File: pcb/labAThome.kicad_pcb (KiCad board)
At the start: 2 copper layers, 100 x 100 mm, 119 parts, among them IC1 MD8002A, J1 I2C, J10 SPK, J11 24.5.GND.3, J12 NEOPIXEL, J13 Power Input 1, J14 Conn_Coaxial, J15 WS2812_OUT, J16 HCP, J2 SRVx, J3 5V, J4 EXT, J5 VPS, J6 FAN2, J7 1wire, J8 1wire, J9 FAN1, K1 G5V-2, K2 G5V-2, K3 G5V-2, M3 SN65HVD230_MODULE, Q1 BC847, Q2 IRLZ44N, Q3 IRLML6344, Q4 BC847, Q5 IRF530, Q6 IRLML5203, SW1 RED, SW2 GREEN, SW4 BLUE, SW5 WHITE, SW7 ROTENC, U1 SR602, U10 MAX3485_MODULE, U11 AM312, U12 24V->4V, U13 LM358, U14 MS4525DO, U15 CCS811_MODULE, U16 24V->5V, U17 DS18B20, U2 TPS5430DDA, U3 Power Input 2, U4 ESP32_DEVKITC_COMPATIBLE, U6 GY-302, U7 Display, U8 MIC, U9 RFM95W-868S2, X1 FAN_6024, m1 Attribution

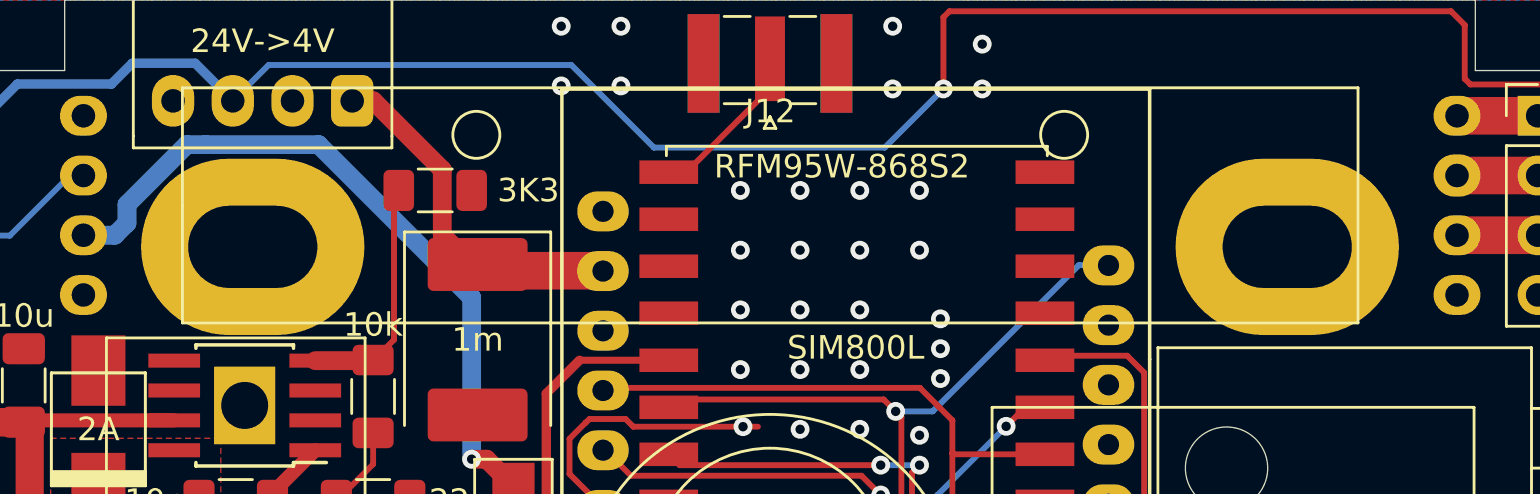
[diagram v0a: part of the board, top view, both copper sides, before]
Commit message: pcb V10 as ordered at JLCPCB
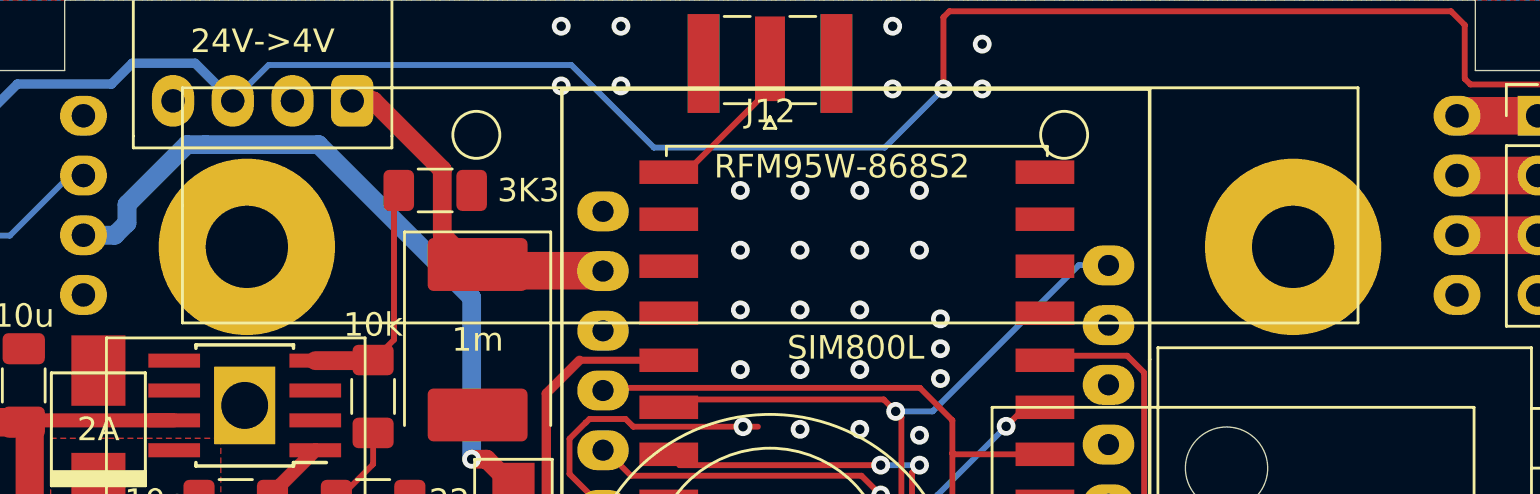
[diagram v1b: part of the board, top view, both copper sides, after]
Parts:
- R11: footprint smopla:Resistor_100W -> liebler_PASSIVES:Resistor_100W
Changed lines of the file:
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@@
     (34 B.Paste user hide)
     (35 F.Paste user hide)
-    (36 B.SilkS user hide)
+    (36 B.SilkS user)
     (37 F.SilkS user)
     (38 B.Mask user hide)
@@
   )
   (setup
-    (last_trace_width 0.4)
+    (last_trace_width 0.25)
     (user_trace_width 0.3)
     (user_trace_width 0.4)
@@
     (add_net /Q2_D)
   )
+  (module liebler_PASSIVES:Resistor_100W (layer B.Cu)
+    (at 80 50.5)
+    (fp_text reference R11 (at -27.5 3.5) (layer B.SilkS) hide
+      (effects (font (size 1 1) (thickness 0.15)) (justify mirror))
+    )
+    (fp_text value "22R, 100W" (at 0 0) (layer B.SilkS)
+      (effects (font (size 4 4) (thickness 0.5)) (justify mirror))
+    )
+    (fp_line (start -30 4.5) (end 30 4.5) (layer B.SilkS) (width 0.12))
+    (fp_line (start 30 7.5) (end 30 -13.5) (layer B.SilkS) (width 0.12))
+    (fp_line (start 30 -13.5) (end -30 -13.5) (layer B.SilkS) (width 0.12))
+    (fp_line (start -30 -13.5) (end -30 7.5) (layer B.SilkS) (width 0.12))
+    (fp_line (start 30 0) (end 30 3) (layer B.SilkS) (width 0.12))
+    (fp_line (start 30 6.5) (end -30 6.5) (layer B.SilkS) (width 0.12))
+    (fp_line (start -30 7.5) (end 30 7.5) (layer B.SilkS) (width 0.12))
+    (fp_line (start 30 5.5) (end -30 5.5) (layer B.SilkS) (width 0.12))
+    (fp_line (start -30 -6.5) (end 30 -6.5) (layer B.SilkS) (width 0.12))
+    (fp_line (start -30 -7.5) (end 30 -7.5) (layer B.SilkS) (width 0.12))
+    (fp_line (start 30 2) (end 38 2) (layer B.SilkS) (width 0.12))
+    (fp_line (start 38 -2) (end 30 -2) (layer B.SilkS) (width 0.12))
+    (fp_line (start -30 -2) (end -38 -2) (layer B.SilkS) (width 0.12))
+    (fp_line (start -38 2) (end -30 2) (layer B.SilkS) (width 0.12))
+    (fp_line (start -30 -5.5) (end 30 -5.5) (layer B.SilkS) (width 0.12))
+    (fp_line (start -30 -4.5) (end 30 -4.5) (layer B.SilkS) (width 0.12))
+    (pad 2 thru_hole circle (at 39.7 0) (size 3.6 3.6) (drill 1.6) (layers *.Cu *.Mask)
+      (net 49 /Q2_D))
+    (pad 1 thru_hole circle (at -39.7 0) (size 3.6 3.6) (drill 1.6) (layers *.Cu *.Mask)
+      (net 2 +24V))
+    (pad "" np_thru_hole oval (at -22.25 -10) (size 7.5 7.5) (drill oval 3.5) (layers *.Cu *.Mask))
+    (pad "" np_thru_hole oval (at 22.25 -10) (size 7.5 7.5) (drill oval 3.5) (layers *.Cu *.Mask))
+    (model "${CUSTOM_LIBS}/smopla.3d/Resistor 100W.stp"
+      (offset (xyz 30 0 27.5))
+      (scale (xyz 1 1 1))
+      (rotate (xyz -90 0 90))
+    )
+    (model "${CUSTOM_LIBS}/smopla.3d/Resistor 100W.stp"
+      (offset (xyz 30 0 49.5))
+      (scale (xyz 1 1 1))
+      (rotate (xyz -90 0 90))
+    )
+  )
   (module liebler_MODULES:PIR_Sensor_SR602 (layer F.Cu)
     (at 80 55.626)
@@
       (effects (font (size 1 1) (thickness 0.15)))
     )
+    (fp_circle (center 0 0) (end 0 -8) (layer F.SilkS) (width 0.12))
+    (fp_circle (center 0 0) (end 0 -8) (layer F.CrtYd) (width 0.12))
     (fp_arc (start 8 0) (end 7.750001 -1.749999) (angle -163.7397953) (layer F.SilkS) (width 0.12))
     (fp_arc (start -8 0) (end -7.750001 1.749999) (angle -164.7448813) (layer F.SilkS) (width 0.12))
-    (fp_circle (center 0 0) (end 0 -8) (layer F.SilkS) (width 0.12))
-    (fp_circle (center 0 0) (end 0 -8) (layer F.CrtYd) (width 0.12))
     (pad 3 thru_hole circle (at 2.54 6.096) (size 1.8 1.8) (drill 1) (layers *.Cu *.Mask)
       (net 38 MOVEMENT))
@@
     (fp_text value ESP32_DEVKITC_COMPATIBLE (at 0 1.5) (layer F.Fab)
       (effects (font (size 1 1) (thickness 0.15)))
-    )
-    (fp_text user "WIFI ANTENNA" (at 0 -24) (layer F.SilkS)
-      (effects (font (size 2 1.5) (thickness 0.15)))
-    )
-    (fp_text user USB (at 0 24) (layer F.SilkS)
-      (effects (font (size 2 1.5) (thickness 0.15)))
     )
     (fp_line (start 0 -27.5) (end 14 -27.5) (layer F.SilkS) (width 0.12))
@@
     (fp_line (start 14 -27.5) (end -14 -27.5) (layer F.CrtYd) (width 0.12))
     (fp_line (start -14 -27.5) (end -14 27.5) (layer F.CrtYd) (width 0.12))
+    (fp_text user "WIFI ANTENNA" (at 0 -24) (layer F.SilkS)
+      (effects (font (size 2 1.5) (thickness 0.15)))
+    )
+    (fp_text user USB (at 0 24) (layer F.SilkS)
+      (effects (font (size 2 1.5) (thickness 0.15)))
+    )
     (pad 38 thru_hole circle (at 12.7 -22.86) (size 1.7 1.7) (drill 1) (layers *.Cu *.Mask)
       (net 1 GND))
@@
       (effects (font (size 1 1) (thickness 0.15)))
     )
-    (fp_text user %R (at 3.6 3.8 90) (layer F.Fab) hide
-      (effects (font (size 1 1) (thickness 0.15)))
-    )
     (fp_line (start -0.5 0) (end 0.5 0) (layer F.SilkS) (width 0.12))
     (fp_line (start 0 -0.5) (end 0 0.5) (layer F.SilkS) (width 0.12))
@@
     (fp_line (start -8.516 -3.516) (end -6.103 -3.516) (layer F.CrtYd) (width 0.12))
     (fp_line (start -6.103 -3.516) (end -6.103 -5.929) (layer F.CrtYd) (width 0.12))
+    (fp_text user %R (at 3.6 3.8 90) (layer F.Fab) hide
+      (effects (font (size 1 1) (thickness 0.15)))
+    )
     (pad A thru_hole roundrect (at -7.5 -2.5 270) (size 2 1.6) (drill 1) (layers *.Cu *.Mask) (roundrect_rratio 0.25)
       (net 57 ROTENC_A))
@@
     )
     (fp_text value WHITE (at 4.75 -7.25) (layer F.SilkS)
-      (effects (font (size 1 1) (thickness 0.15)))
-    )
-    (fp_text user %R (at 0.1 0.04) (layer F.Fab) hide
       (effects (font (size 1 1) (thickness 0.15)))
     )
@@
     (fp_line (start 6.15 3.43) (end 6.15 6.15) (layer F.SilkS) (width 0.12))
     (fp_line (start 6.15 -6.15) (end 6.15 -3.43) (layer F.SilkS) (width 0.12))
+    (fp_text user %R (at 0.1 0.04) (layer F.Fab) hide
+      (effects (font (size 1 1) (thickness 0.15)))
+    )
     (pad 2 thru_hole oval (at -6.25 2.5 180) (size 3.048 1.85) (drill 1.3) (layers *.Cu *.Mask)
       (net 6 +5V))
@@
     )
     (fp_text value BLUE (at -0.25 7) (layer F.SilkS)
-      (effects (font (size 1 1) (thickness 0.15)))
-    )
-    (fp_text user %R (at 0.1 0.04) (layer F.Fab) hide
       (effects (font (size 1 1) (thickness 0.15)))
     )
@@
     (fp_line (start 6.15 3.43) (end 6.15 6.15) (layer F.SilkS) (width 0.12))
     (fp_line (start 6.15 -6.15) (end 6.15 -3.43) (layer F.SilkS) (width 0.12))
+    (fp_text user %R (at 0.1 0.04) (layer F.Fab) hide
+      (effects (font (size 1 1) (thickness 0.15)))
+    )
     (pad 2 thru_hole oval (at -6.25 2.5 180) (size 3.048 1.85) (drill 1.3) (layers *.Cu *.Mask)
       (net 6 +5V))
@@
     )
     (fp_text value GREEN (at -7 -6 180) (layer F.SilkS)
-      (effects (font (size 1 1) (thickness 0.15)))
-    )
-    (fp_text user %R (at 0.1 0.04 90) (layer F.Fab) hide
       (effects (font (size 1 1) (thickness 0.15)))
     )
@@
     (fp_line (start 6.15 3.43) (end 6.15 6.15) (layer F.SilkS) (width 0.12))
     (fp_line (start 6.15 -6.15) (end 6.15 -3.43) (layer F.SilkS) (width 0.12))
+    (fp_text user %R (at 0.1 0.04 90) (layer F.Fab) hide
+      (effects (font (size 1 1) (thickness 0.15)))
+    )
     (pad 2 thru_hole oval (at -6.25 2.5 270) (size 3.048 1.85) (drill 1.3) (layers *.Cu *.Mask)
       (net 62 "Net-(R19-Pad2)"))
@@
     )
     (fp_text value RED (at -7 -5.25 180) (layer F.SilkS)
-      (effects (font (size 1 1) (thickness 0.15)))
-    )
-    (fp_text user %R (at 0.1 0.04 90) (layer F.Fab) hide
       (effects (font (size 1 1) (thickness 0.15)))
     )
@@
     (fp_line (start 6.15 3.43) (end 6.15 6.15) (layer F.SilkS) (width 0.12))
     (fp_line (start 6.15 -6.15) (end 6.15 -3.43) (layer F.SilkS) (width 0.12))
+    (fp_text user %R (at 0.1 0.04 90) (layer F.Fab) hide
+      (effects (font (size 1 1) (thickness 0.15)))
+    )
     (pad 2 thru_hole oval (at -6.25 2.5 270) (size 3.048 1.85) (drill 1.3) (layers *.Cu *.Mask)
       (net 62 "Net-(R19-Pad2)"))
@@
     )
   )
-  (module smopla:Resistor_100W (layer B.Cu)
-    (at 80 50.5)
-    (fp_text reference R11 (at 0.01 -0.081) (layer B.SilkS) hide
-      (effects (font (size 1 1) (thickness 0.15)) (justify mirror))
-    )
-    (fp_text value "22R, 100W" (at 25.918 3.856) (layer B.SilkS)
-      (effects (font (size 1 1) (thickness 0.15)) (justify mirror))
-    )
-    (fp_line (start -30 4.5) (end 30 4.5) (layer B.SilkS) (width 0.12))
-    (fp_line (start 30 7.5) (end 30 -13.5) (layer B.SilkS) (width 0.12))
-    (fp_line (start 30 -13.5) (end -30 -13.5) (layer B.SilkS) (width 0.12))
-    (fp_line (start -30 -13.5) (end -30 7.5) (layer B.SilkS) (width 0.12))
-    (fp_line (start 30 0) (end 30 3) (layer B.SilkS) (width 0.12))
-    (fp_line (start 30 6.5) (end -30 6.5) (layer B.SilkS) (width 0.12))
-    (fp_line (start -30 7.5) (end 30 7.5) (layer B.SilkS) (width 0.12))
-    (fp_line (start 30 5.5) (end -30 5.5) (layer B.SilkS) (width 0.12))
-    (fp_line (start -30 -6.5) (end 30 -6.5) (layer B.SilkS) (width 0.12))
-    (fp_line (start -30 -7.5) (end 30 -7.5) (layer B.SilkS) (width 0.12))
-    (fp_line (start 30 2) (end 38 2) (layer B.SilkS) (width 0.12))
-    (fp_line (start 38 -2) (end 30 -2) (layer B.SilkS) (width 0.12))
-    (fp_line (start -30 -2) (end -38 -2) (layer B.SilkS) (width 0.12))
-    (fp_line (start -38 2) (end -30 2) (layer B.SilkS) (width 0.12))
-    (fp_line (start -30 -5.5) (end 30 -5.5) (layer B.SilkS) (width 0.12))
-    (fp_line (start -30 -4.5) (end 30 -4.5) (layer B.SilkS) (width 0.12))
-    (pad 2 thru_hole circle (at 39.7 0) (size 3.6 3.6) (drill 1.6) (layers *.Cu *.Mask)
-      (net 49 /Q2_D))
-    (pad 1 thru_hole circle (at -39.7 0) (size 3.6 3.6) (drill 1.6) (layers *.Cu *.Mask)
-      (net 2 +24V))
-    (pad "" thru_hole oval (at -22 -10) (size 9.5 7.5) (drill oval 5.5 3.5) (layers *.Cu *.Mask))
-    (pad "" thru_hole oval (at 22 -10) (size 9.5 7.5) (drill oval 5.5 3.5) (layers *.Cu *.Mask))
-    (model "${CUSTOM_LIBS}/smopla.3d/Resistor 100W.stp"
-      (offset (xyz 30 0 27.5))
-      (scale (xyz 1 1 1))
-      (rotate (xyz -90 0 90))
-    )
-    (model "${CUSTOM_LIBS}/smopla.3d/Resistor 100W.stp"
-      (offset (xyz 30 0 49.5))
-      (scale (xyz 1 1 1))
-      (rotate (xyz -90 0 90))
-    )
-  )
